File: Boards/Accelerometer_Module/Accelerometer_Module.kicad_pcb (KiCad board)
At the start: 2 copper layers, 66.2 x 66.2 mm, 54 parts, among them J1 CONN_02X03, J2 SD_socket, SW1 SW_Push_SPST_NO, U1 ATmega328P-AU, U101 TPS560430YF, U2 LIS3DHTR, U3 INA260

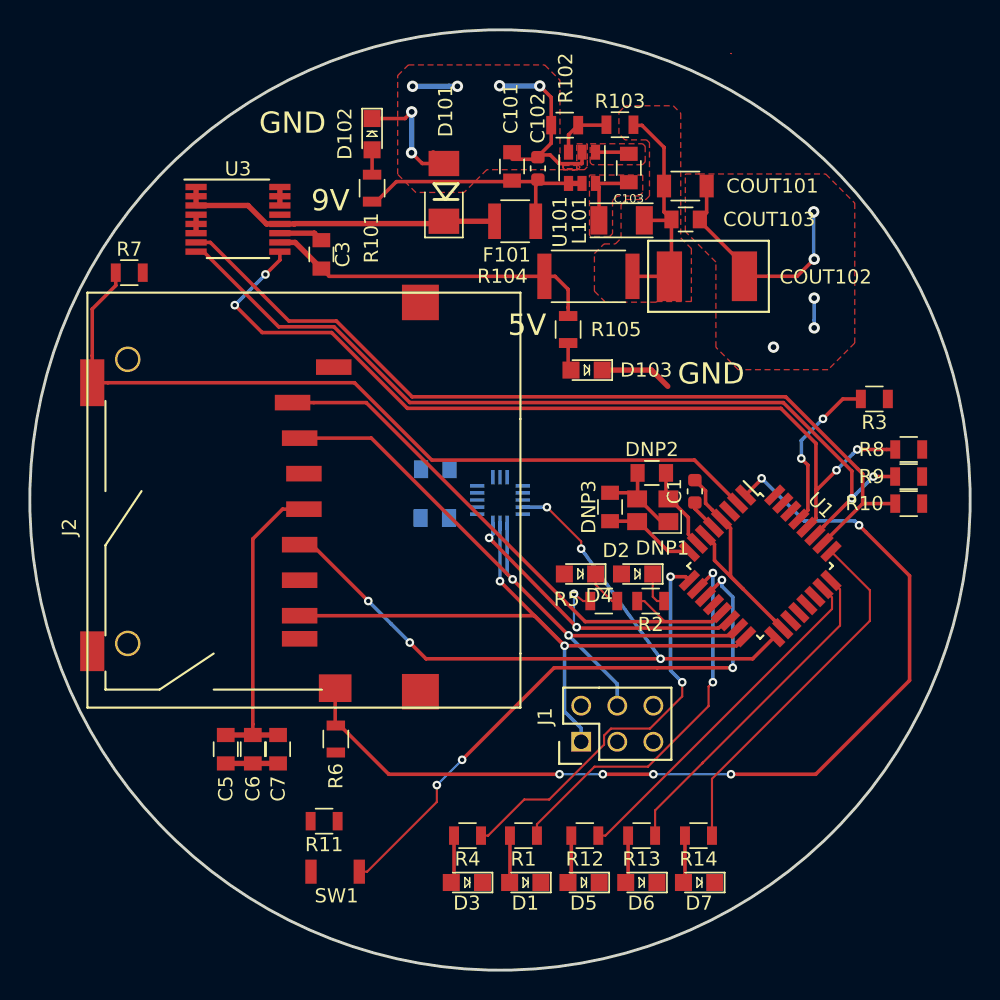
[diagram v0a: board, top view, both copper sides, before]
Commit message: Editing Layout
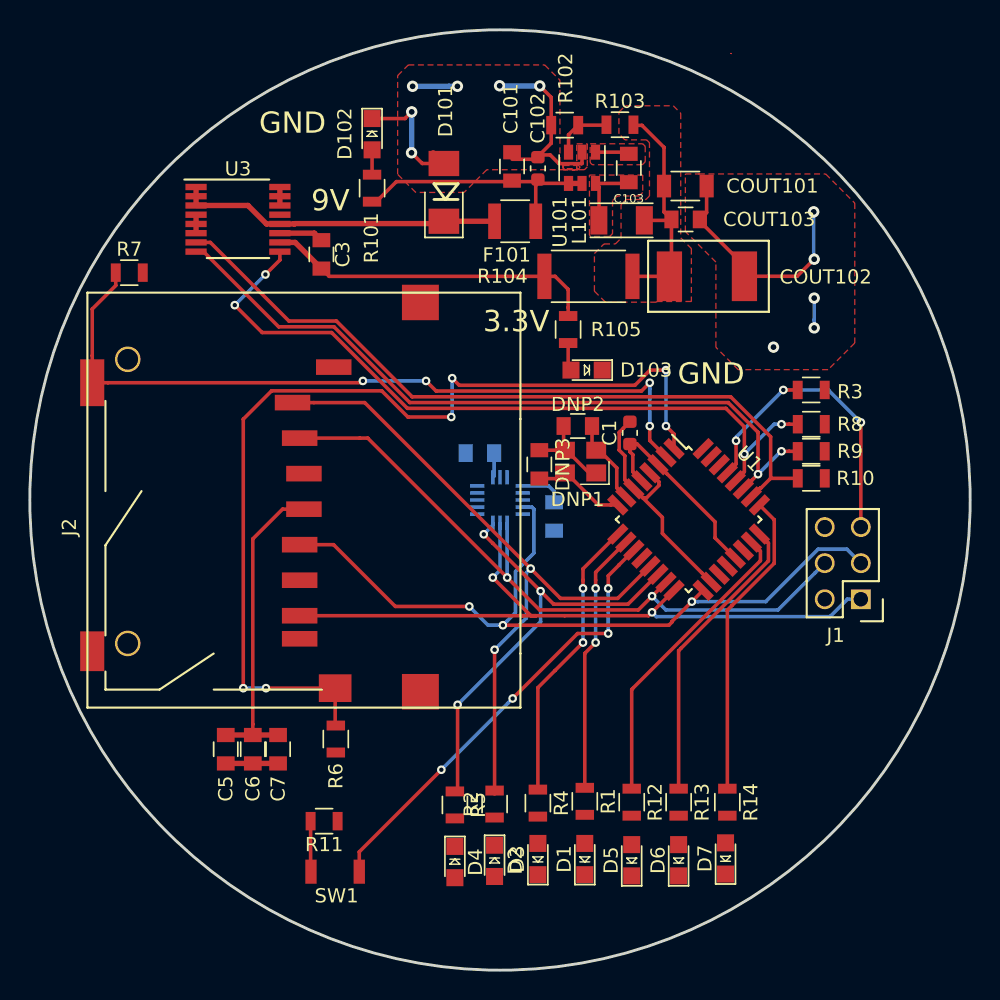
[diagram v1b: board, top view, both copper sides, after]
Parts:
- moved D2 22.5 mm to (72.3, 143.3), turned to 270 degrees
- moved D4 22.1 mm to (69.5, 143.3), turned to 270 degrees
- moved J1 22.1 mm to (98.0, 124.8), turned to 180 degrees
- moved R2 18.0 mm to (72.3, 139.3), turned to 90 degrees
- moved R5 17.8 mm to (69.5, 139.3), turned to 270 degrees
- moved C2 9.00 mm to (76.5, 119.0), turned to 90 degrees
- moved R10 7.08 mm to (94.6, 116.3)
- moved R8 7.08 mm to (94.6, 112.5)
- moved R9 7.08 mm to (94.5, 114.4)
- moved DNP2 6.17 mm to (78.1, 112.6)
- moved C1 6.15 mm to (81.8, 113.1)
- moved DNP1 6.13 mm to (78.3, 115.2)
- moved U1 6.01 mm to (85.9, 119.2)
- moved DNP3 5.81 mm to (75.4, 115.4)
- moved C4 5.57 mm to (71.2, 114.6), turned to 180 degrees
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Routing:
- net /RESET: track 11.4 -> 22.6 mm, vias 2 -> 3
- net /SCL: track 63.0 -> 53.2 mm
- net /ALERT: track 62.0 -> 52.8 mm
- net /CS_SD: track 39.8 -> 48.7 mm, vias 0 -> 2
- net Net-(R1-Pad1): track 27.4 -> 18.5 mm
- net Net-(SW1-Pad1): track 41.1 -> 32.4 mm
- net Net-(R4-Pad1): track 28.8 -> 20.3 mm
- net /SDA: track 61.8 -> 53.4 mm
- net /CS: track 24.7 -> 33.1 mm
- net VCC: track 41.4 -> 49.8 mm
- net GND: track 70.0 -> 76.6 mm
- net /PC2: track 25.7 -> 21.8 mm
- net /SCK: track 52.6 -> 56.4 mm, vias 5 -> 3
- net /Detect: track 57.7 -> 54.2 mm, vias 0 -> 4
- net Net-(D5-Pad2): track 3.40 -> 0.00 mm
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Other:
- board text added: "3.3V"
- board text removed: "5V"
